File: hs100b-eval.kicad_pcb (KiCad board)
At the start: 2 copper layers, 60 x 50 mm, 42 parts, among them IC1 HS-100B, J1 SPKR, J2 MIC, J3 RADIO_DATA, SW1 MUTE_REC, SW2 MUTE_PLAY, SW3 VOL_DN, SW4 VOL_UP

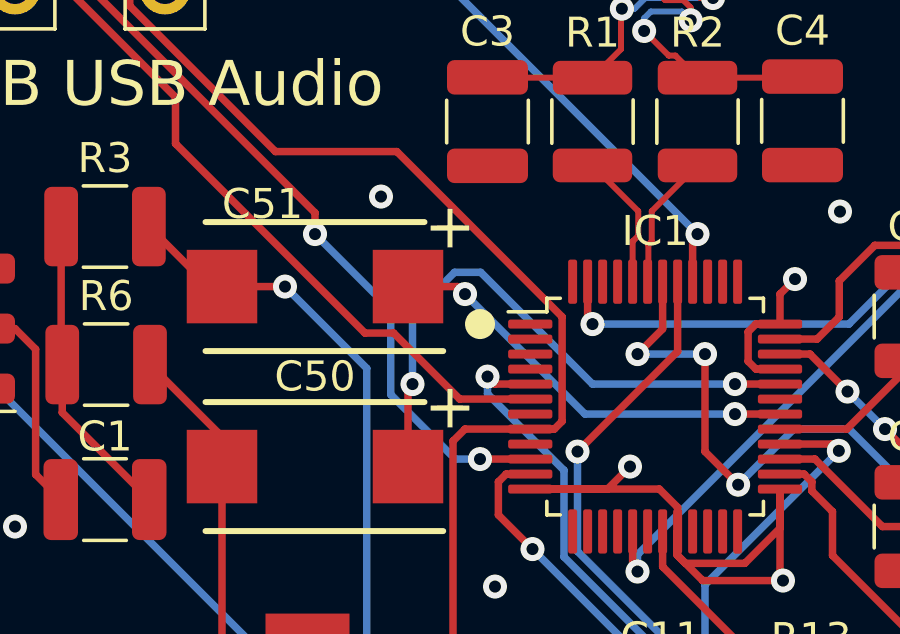
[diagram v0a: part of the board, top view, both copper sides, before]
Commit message: Update BOM
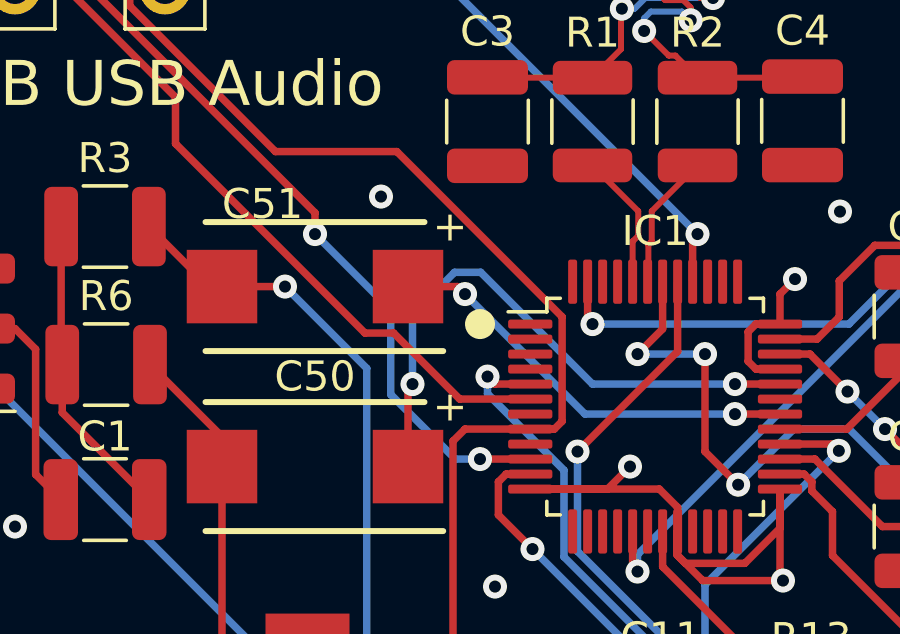
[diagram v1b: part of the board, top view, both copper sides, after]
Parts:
- C50, C51: footprint 293D477X9010E2TE3:CAPPM7343X430N -> Vishay:CAPPM7343X430N
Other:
- board text removed: "+"
